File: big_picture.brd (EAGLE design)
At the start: 160 x 100 mm, 13 parts, among them K1 RELAY-SPDT-JZC-11F, M1 MOTOR10MM

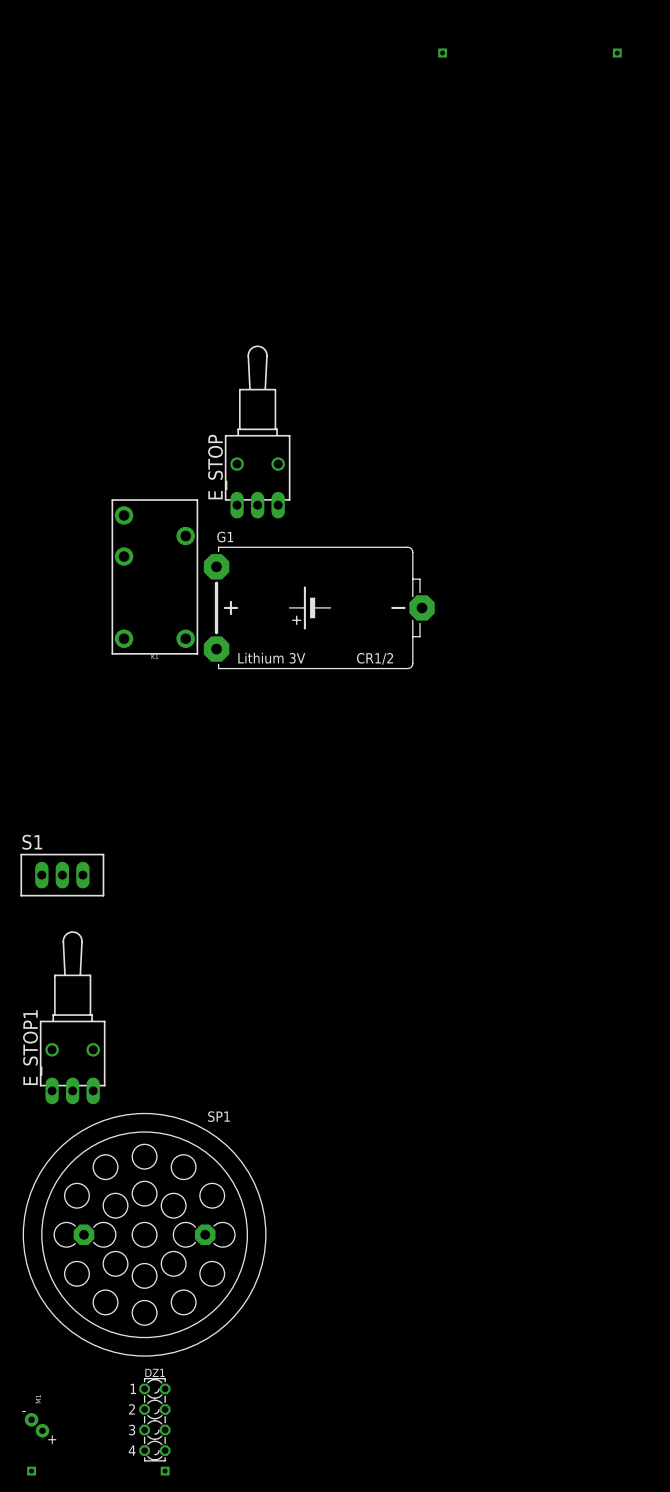
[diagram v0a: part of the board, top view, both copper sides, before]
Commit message: redid general schematic
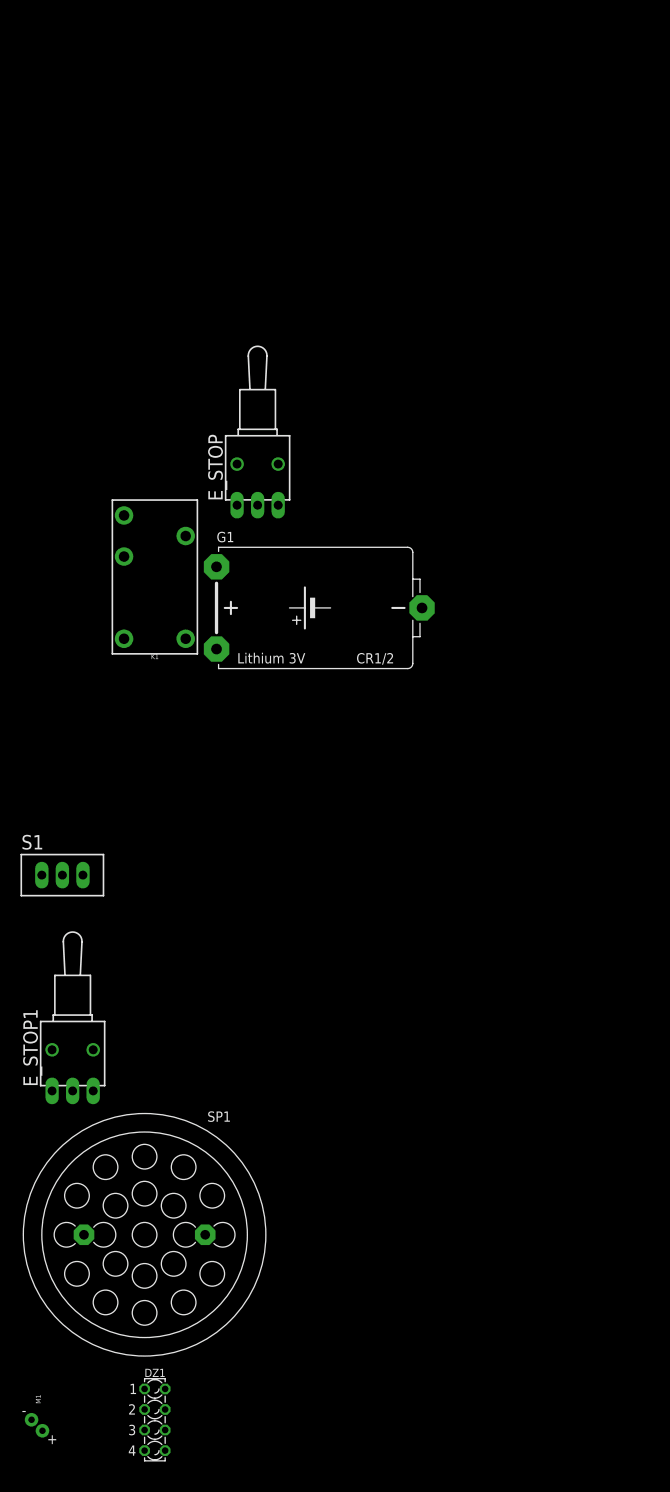
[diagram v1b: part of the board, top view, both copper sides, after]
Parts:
- removed U$4: BUCK, big_picture_parts:BUCK
- removed U$5: AUX, big_picture_parts:AUX
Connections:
- new net N$2: DZ1.A1
- new net N$8: DZ1.A3
- new net N$9: DZ1.A2
- net N$1: no longer U$4.P$2
- net N$31: no longer DZ1.A1, DZ1.A2, DZ1.A3, DZ1.A4, M1.+, U$5.P$1
- net N$35: no longer U$4.P$1
- net N$5: now also M1.+; no longer U$5.P$2
- net PDB_GND: no longer DZ1.K4
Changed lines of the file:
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@@
 <element name="U$2" library="big_picture_parts" package="BUCK" value="" x="-8.89" y="-24.13"/>
 <element name="U$3" library="big_picture_parts" package="HORN" value="" x="0" y="-34.29"/>
-<element name="U$4" library="big_picture_parts" package="BUCK" value="BUCK" x="-74.93" y="-27.94">
-<attribute name="BUCK" value="" x="-74.93" y="-27.94" size="1.778" layer="27" display="off"/>
-</element>
 <element name="E_STOP" library="switch" library_urn="urn:adsk.eagle:library:380" package="TL3XWO" package3d_urn="urn:adsk.eagle:package:27754/1" value="TL36WO" x="-110.49" y="-77.47">
 <attribute name="NAME" x="-114.808" y="-82.042" size="1.778" layer="25" rot="R90"/>
@@
 <element name="S1" library="switch" library_urn="urn:adsk.eagle:library:380" package="TL3XPO" package3d_urn="urn:adsk.eagle:package:27745/1" value="TL37PO" x="-134.62" y="-128.27"/>
 <element name="E_STOP1" library="switch" library_urn="urn:adsk.eagle:library:380" package="TL3XWO" package3d_urn="urn:adsk.eagle:package:27754/1" value="TL36WO" x="-133.35" y="-149.86"/>
-<element name="U$5" library="big_picture_parts" package="AUX" value="AUX" x="-128.27" y="-201.93">
-<attribute name="AUX" value="" x="-128.27" y="-157.48" size="1.778" layer="27" display="off"/>
-</element>
 <element name="SP1" library="buzzer" library_urn="urn:adsk.eagle:library:113" package="AL30P" package3d_urn="urn:adsk.eagle:package:5288/1" value="AL30P" x="-124.46" y="-172.72">
 <attribute name="MF" value="" x="-124.46" y="-175.26" size="1.778" layer="27" display="off"/>
@@
 <contactref element="K1" pad="2"/>
 <contactref element="S1" pad="3"/>
-<contactref element="U$4" pad="P$1"/>
 <wire x1="-132.08" y1="-128.27" x2="-127" y2="-88.9" width="0" layer="19" extent="1-1"/>
-<wire x1="-87.63" y1="-26.67" x2="-127" y2="-88.9" width="0" layer="19" extent="1-1"/>
 </signal>
 <signal name="N$1">
-<contactref element="U$4" pad="P$2"/>
 <contactref element="E_STOP1" pad="2"/>
-<wire x1="-133.35" y1="-154.94" x2="-66.04" y2="-26.67" width="0" layer="19" extent="1-1"/>
 </signal>
 <signal name="N$3">
@@
 <wire x1="-113.03" y1="-82.55" x2="-119.38" y2="-86.36" width="0" layer="19" extent="1-1"/>
 </signal>
-<signal name="N$2">
-<contactref element="G1" pad="-"/>
-</signal>
 <signal name="N$31">
-<contactref element="U$5" pad="P$1"/>
 <contactref element="SP1" pad="2"/>
-<contactref element="M1" pad="+"/>
-<contactref element="DZ1" pad="A1"/>
-<contactref element="DZ1" pad="A2"/>
-<contactref element="DZ1" pad="A4"/>
-<contactref element="DZ1" pad="A3"/>
-<wire x1="-137.08" y1="-196.94" x2="-138.43" y2="-201.93" width="0" layer="19" extent="1-1"/>
-<wire x1="-124.46" y1="-196.85" x2="-137.08" y2="-196.94" width="0" layer="19" extent="1-1"/>
-<wire x1="-124.46" y1="-199.39" x2="-124.46" y2="-196.85" width="0" layer="19" extent="1-1"/>
-<wire x1="-124.46" y1="-194.31" x2="-124.46" y2="-196.85" width="0" layer="19" extent="1-1"/>
-<wire x1="-124.46" y1="-191.77" x2="-124.46" y2="-194.31" width="0" layer="19" extent="1-1"/>
-<wire x1="-116.967" y1="-172.72" x2="-124.46" y2="-191.77" width="0" layer="19" extent="1-1"/>
-</signal>
-<signal name="N$5">
-<contactref element="U$5" pad="P$2"/>
 </signal>
 <signal name="PDB_GND">
@@
 <contactref element="DZ1" pad="K2"/>
 <contactref element="DZ1" pad="K3"/>
-<contactref element="DZ1" pad="K4"/>
 <wire x1="-121.92" y1="-196.85" x2="-138.43" y2="-195.58" width="0" layer="19" extent="1-1"/>
-<wire x1="-121.92" y1="-199.39" x2="-121.92" y2="-196.85" width="0" layer="19" extent="1-1"/>
 <wire x1="-121.92" y1="-194.31" x2="-121.92" y2="-196.85" width="0" layer="19" extent="1-1"/>
 <wire x1="-121.92" y1="-191.77" x2="-121.92" y2="-194.31" width="0" layer="19" extent="1-1"/>
 <wire x1="-131.953" y1="-172.72" x2="-121.92" y2="-191.77" width="0" layer="19" extent="1-1"/>
 </signal>
+<signal name="N$4">
+<contactref element="G1" pad="-"/>
+</signal>
+<signal name="N$2">
+<contactref element="DZ1" pad="A1"/>
+</signal>
+<signal name="N$5">
+<contactref element="M1" pad="+"/>
+</signal>
+<signal name="N$8">
+<contactref element="DZ1" pad="A3"/>
+</signal>
+<signal name="N$9">
+<contactref element="DZ1" pad="A2"/>
+</signal>
 </signals>
